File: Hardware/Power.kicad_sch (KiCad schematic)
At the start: 37 parts, among them U11 AP2112K-3.3, U5 AP2112K-3.3, U6 REC15E-2405SZ, U7 Ag9905M

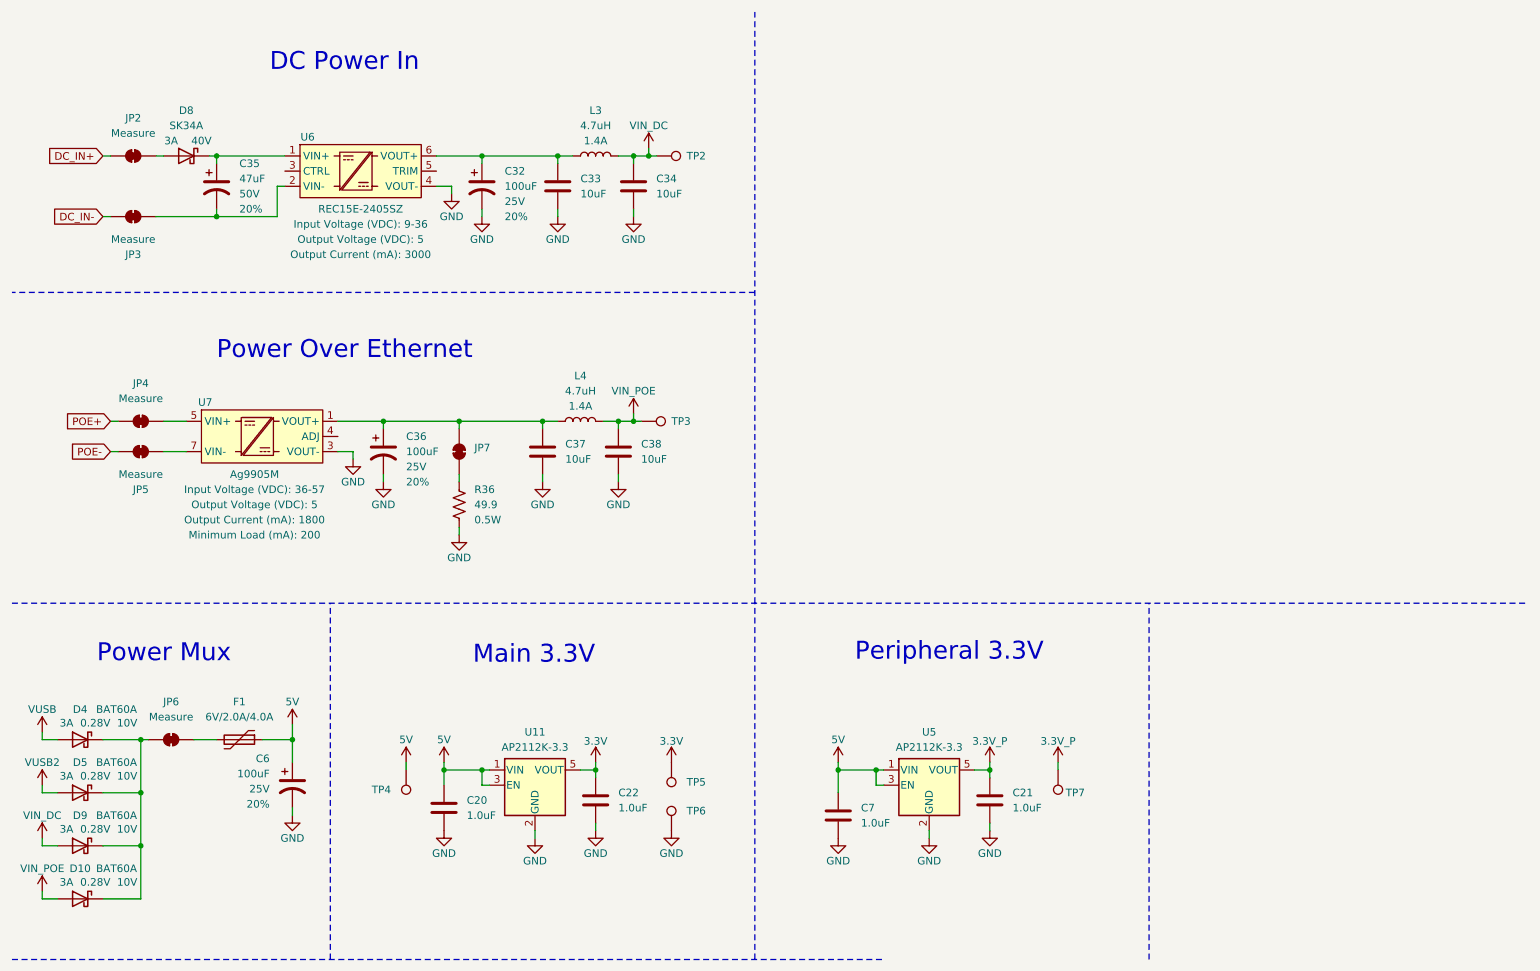
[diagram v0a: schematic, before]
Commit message: More WIP
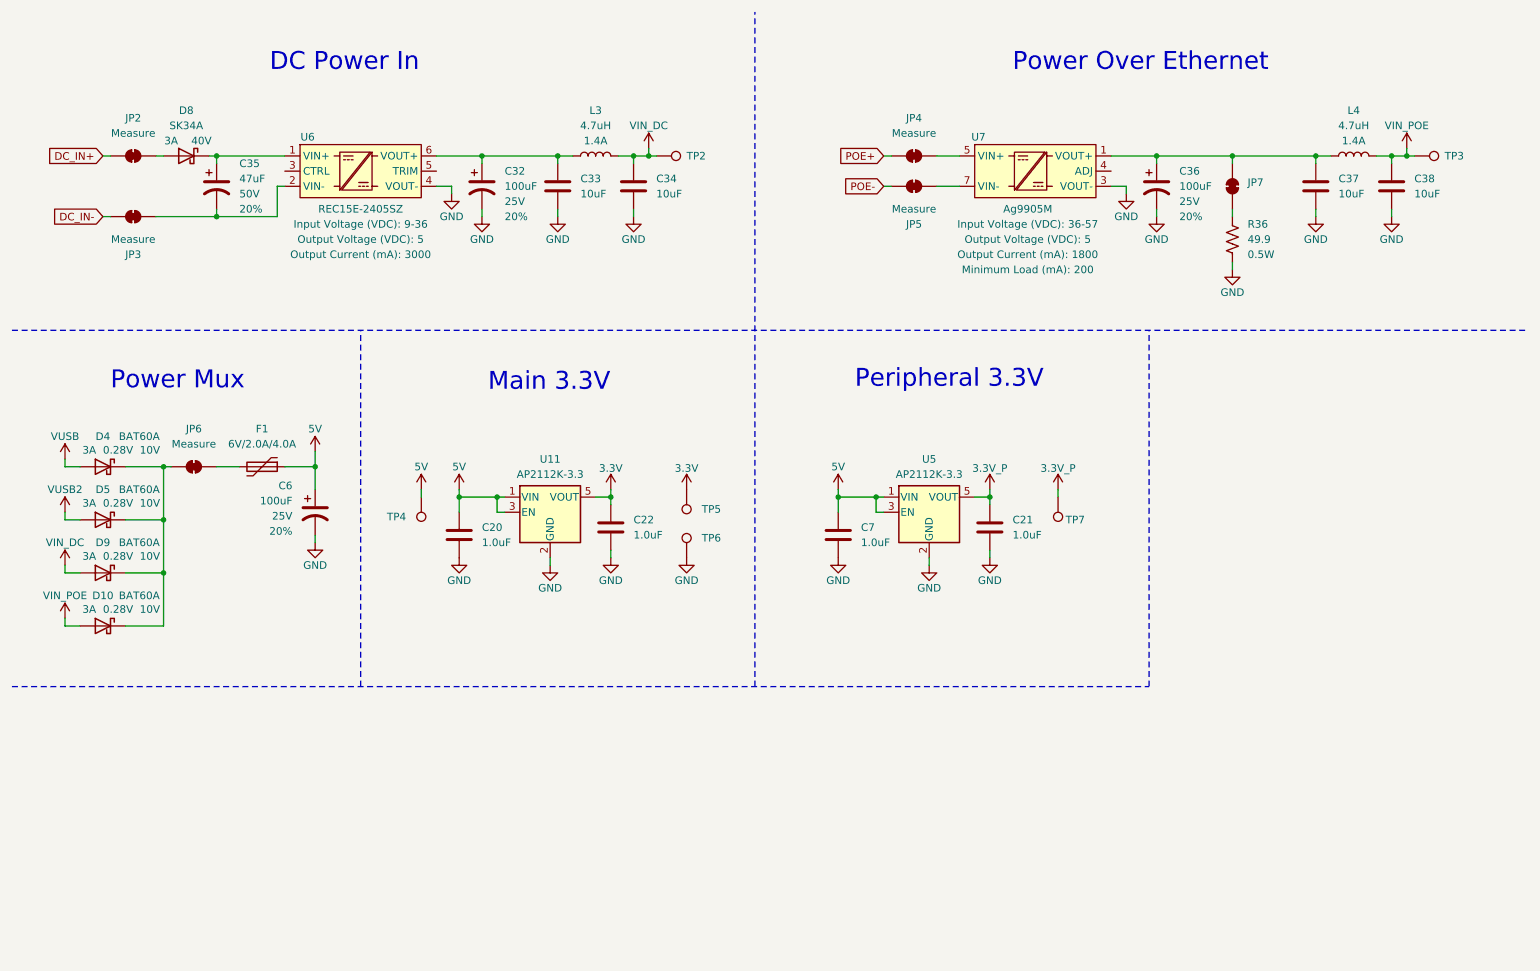
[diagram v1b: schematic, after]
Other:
- moved on the sheet: C20, C21, C22, C36, C37, C38, C6, C7, D10, D4, D5, D9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
